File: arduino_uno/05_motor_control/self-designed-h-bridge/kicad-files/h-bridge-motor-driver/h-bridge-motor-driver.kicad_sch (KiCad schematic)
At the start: 21 parts, among them J1 Conn_01x05_Pin, J3 2601-3102, J4 2601-3102, Q1 IRF9540N, Q2 IRLIZ44N, Q3 IRF9540N, Q4 IRLIZ44N, Q5 BC547, Q6 BC547

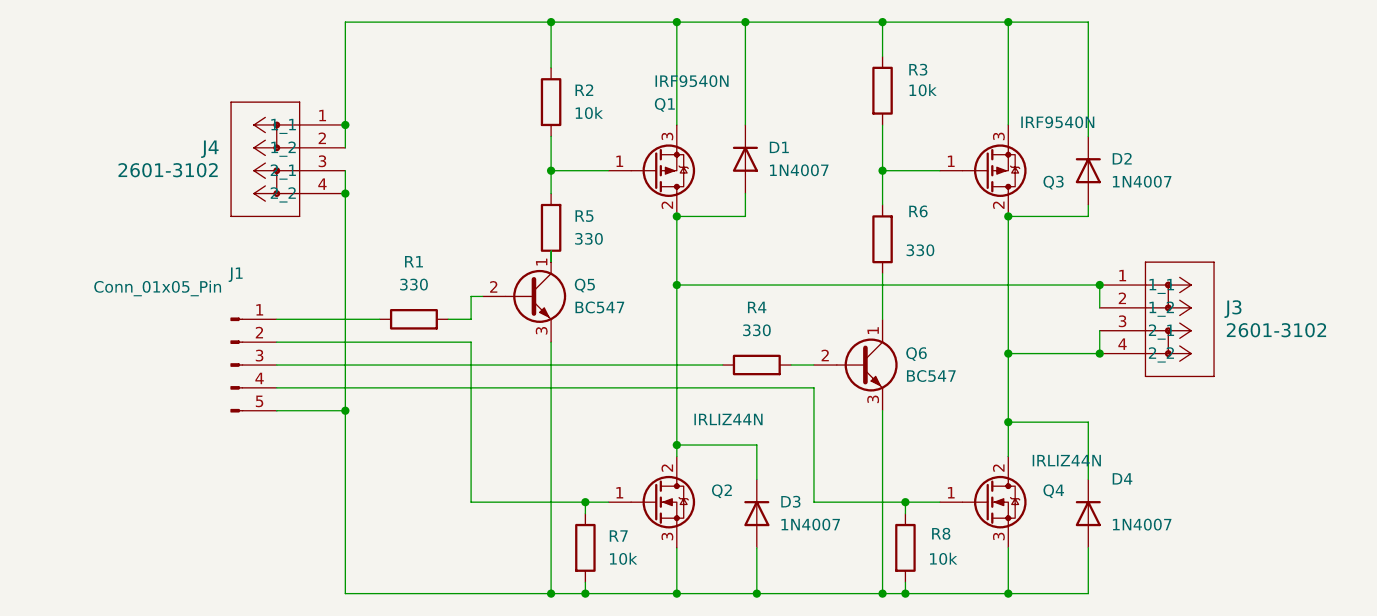
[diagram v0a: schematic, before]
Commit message: start routing
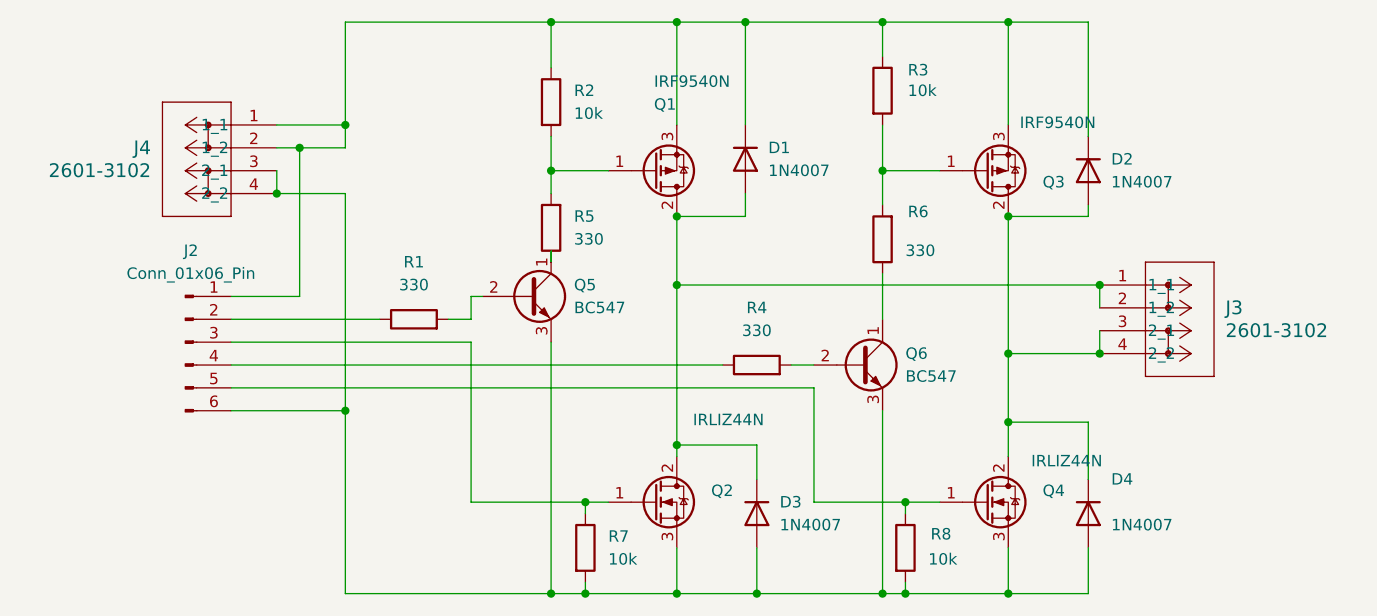
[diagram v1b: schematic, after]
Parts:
- removed J1: Conn_01x05_Pin, Connector_PinHeader_2.54mm:PinHeader_1x05_P2.54mm_Vertical, symbol Connector:Conn_01x05_Pin
- added J2: Conn_01x06_Pin, Connector_PinSocket_2.54mm:PinSocket_1x06_P2.54mm_Vertical, symbol Connector:Conn_01x06_Pin
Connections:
- net at D1.1 (K), D2.1 (K), J4.1 (1_1)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: now also J2.1 (Pin_1)
- net at Q4.1 (G), R8.1: now also J2.5 (Pin_5)
- net at D3.2 (A), D4.2 (A), J4.3 (2_1)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: now also J2.6 (Pin_6)
- net at Q2.1 (G), R7.1: now also J2.3 (Pin_3)
- net at R1.1: now also J2.2 (Pin_2)
- net at R4.1: now also J2.4 (Pin_4)
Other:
- moved on the sheet: J4
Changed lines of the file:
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@@
 	(paper "A4")
 	(junction
+		(at 66.04 60.96)
+		(diameter 0)
+		(color 0 0 0 0)
+	)
+	(junction
 		(at 97.79 100.33)
 		(diameter 0)
@@
 	)
 	(junction
-		(at 71.12 66.04)
-		(diameter 0)
-		(color 0 0 0 0)
-	)
-	(junction
 		(at 107.95 110.49)
 		(diameter 0)
@@
 	)
 	(junction
+		(at 63.5 66.04)
+		(diameter 0)
+		(color 0 0 0 0)
+	)
+	(junction
 		(at 107.95 93.98)
 		(diameter 0)
@@
 	(wire
 		(pts
+			(xy 58.42 87.63) (xy 123.19 87.63)
+		)
+		(stroke
+			(width 0)
+			(type default)
+		)
+	)
+	(wire
+		(pts
 			(xy 93.98 63.5) (xy 93.98 66.04)
 		)
@@
 	(wire
 		(pts
+			(xy 63.5 60.96) (xy 66.04 60.96)
+		)
+		(stroke
+			(width 0)
+			(type default)
+		)
+	)
+	(wire
+		(pts
 			(xy 85.09 77.47) (xy 85.09 80.01)
 		)
@@
 	(wire
 		(pts
+			(xy 63.5 58.42) (xy 71.12 58.42)
+		)
+		(stroke
+			(width 0)
+			(type default)
+		)
+	)
+	(wire
+		(pts
 			(xy 130.81 58.42) (xy 130.81 63.5)
 		)
@@
 	(wire
 		(pts
+			(xy 58.42 85.09) (xy 113.03 85.09)
+		)
+		(stroke
+			(width 0)
+			(type default)
+		)
+	)
+	(wire
+		(pts
 			(xy 130.81 63.5) (xy 137.16 63.5)
 		)
@@
 	(wire
 		(pts
+			(xy 58.42 82.55) (xy 85.09 82.55)
+		)
+		(stroke
+			(width 0)
+			(type default)
+		)
+	)
+	(wire
+		(pts
 			(xy 97.79 101.6) (xy 97.79 100.33)
 		)
@@
 	(wire
 		(pts
+			(xy 58.42 90.17) (xy 71.12 90.17)
+		)
+		(stroke
+			(width 0)
+			(type default)
+		)
+	)
+	(wire
+		(pts
 			(xy 85.09 100.33) (xy 97.79 100.33)
 		)
@@
 	(wire
 		(pts
+			(xy 63.5 66.04) (xy 71.12 66.04)
+		)
+		(stroke
+			(width 0)
+			(type default)
+		)
+	)
+	(wire
+		(pts
 			(xy 154.94 76.2) (xy 154.94 78.74)
 		)
@@
 	(wire
 		(pts
+			(xy 66.04 60.96) (xy 66.04 77.47)
+		)
+		(stroke
+			(width 0)
+			(type default)
+		)
+	)
+	(wire
+		(pts
 			(xy 116.84 110.49) (xy 107.95 110.49)
 		)
@@
 	(wire
 		(pts
-			(xy 63.5 90.17) (xy 71.12 90.17)
-		)
-		(stroke
-			(width 0)
-			(type default)
-		)
-	)
-	(wire
-		(pts
 			(xy 144.78 105.41) (xy 144.78 110.49)
 		)
@@
 	(wire
 		(pts
-			(xy 63.5 80.01) (xy 74.93 80.01)
-		)
-		(stroke
-			(width 0)
-			(type default)
-		)
-	)
-	(wire
-		(pts
-			(xy 63.5 85.09) (xy 113.03 85.09)
+			(xy 58.42 77.47) (xy 66.04 77.47)
 		)
 		(stroke
@@
 	(wire
 		(pts
-			(xy 71.12 58.42) (xy 71.12 60.96)
-		)
-		(stroke
-			(width 0)
-			(type default)
-		)
-	)
-	(wire
-		(pts
 			(xy 144.78 46.99) (xy 153.67 46.99)
 		)
@@
 	(wire
 		(pts
-			(xy 63.5 82.55) (xy 85.09 82.55)
-		)
-		(stroke
-			(width 0)
-			(type default)
-		)
-	)
-	(wire
-		(pts
 			(xy 116.84 93.98) (xy 107.95 93.98)
 		)
@@
 	(wire
 		(pts
-			(xy 71.12 63.5) (xy 71.12 66.04)
+			(xy 63.5 63.5) (xy 63.5 66.04)
 		)
 		(stroke
@@
 	(wire
 		(pts
+			(xy 71.12 60.96) (xy 71.12 58.42)
+		)
+		(stroke
+			(width 0)
+			(type default)
+		)
+	)
+	(wire
+		(pts
+			(xy 66.04 60.96) (xy 71.12 60.96)
+		)
+		(stroke
+			(width 0)
+			(type default)
+		)
+	)
+	(wire
+		(pts
 			(xy 144.78 110.49) (xy 133.35 110.49)
 		)
@@
 	(wire
 		(pts
-			(xy 63.5 87.63) (xy 123.19 87.63)
+			(xy 58.42 80.01) (xy 74.93 80.01)
 		)
 		(stroke
@@
 	)
 	(symbol
-		(lib_id "Connector:Conn_01x05_Pin")
-		(at 58.42 85.09 0)
-		(unit 1)
-		(exclude_from_sim no)
-		(in_bom yes)
-		(on_board yes)
-		(dnp no)
-		(property "Reference" "J1"
-			(at 59.055 74.93 0)
-			(effects
-				(font
-					(size 1.27 1.27)
-				)
-			)
-		)
-		(property "Value" "Conn_01x05_Pin"
-			(at 50.292 76.454 0)
-			(effects
-				(font
-					(size 1.27 1.27)
-				)
-			)
-		)
-		(property "Footprint" "Connector_PinHeader_2.54mm:PinHeader_1x05_P2.54mm_Vertical"
-			(at 58.42 85.09 0)
-			(effects
-				(font
-					(size 1.27 1.27)
-				)
-				(hide yes)
-			)
-		)
-		(property "Datasheet" "~"
-			(at 58.42 85.09 0)
-			(effects
-				(font
-					(size 1.27 1.27)
-				)
-				(hide yes)
-			)
-		)
-		(property "Description" "Generic connector, single row, 01x05, script generated"
-			(at 58.42 85.09 0)
-			(effects
-				(font
-					(size 1.27 1.27)
-				)
-				(hide yes)
-			)
-		)
-		(pin "2"
-		)
-		(pin "5"
-		)
-		(pin "3"
-		)
-		(pin "1"
-		)
-		(pin "4"
-		)
-		(instances
-			(project ""
-				(path "/c86b6916-14ad-4ba0-a61b-f63bb8896688"
-					(reference "J1")
-					(unit 1)
-				)
-			)
-		)
-	)
-	(symbol
 		(lib_id "Transistor_BJT:BC547")
 		(at 128.27 85.09 0)
@@
 		(lib_name "2601-3102_1")
 		(lib_id "Wago 2601-3102:2601-3102")
-		(at 71.12 58.42 0)
+		(at 63.5 58.42 0)
 		(mirror y)
 		(unit 1)
@@
 		(dnp no)
 		(property "Reference" "J4"
-			(at 57.15 60.9599 0)
+			(at 49.53 60.9599 0)
 			(effects
 				(font
@@
 		)
 		(property "Value" "2601-3102"
-			(at 57.15 63.4999 0)
+			(at 49.53 63.4999 0)
 			(effects
 				(font
@@
 		)
 		(property "Footprint" "WAGO 2601-3102:CONN2_2601-3102_WAG"
-			(at 71.12 58.42 0)
+			(at 63.5 58.42 0)
 			(effects
 				(font
@@
 		)
 		(property "Datasheet" "2601-3102"
-			(at 71.12 58.42 0)
+			(at 63.5 58.42 0)
 			(effects
 				(font
@@
 		)
 		(property "Description" ""
-			(at 71.12 58.42 0)
+			(at 63.5 58.42 0)
 			(effects
 				(font
@@
 					(unit 1)
 				)
+			)
+		)
+	)
+	(symbol
+		(lib_id "Connector:Conn_01x06_Pin")
+		(at 53.34 82.55 0)
+		(unit 1)
+		(exclude_from_sim no)
+		(in_bom yes)
+		(on_board yes)
+		(dnp no)
+		(fields_autoplaced yes)
+		(property "Reference" "J2"
+			(at 53.975 72.39 0)
+			(effects
+				(font
+					(size 1.27 1.27)
+				)
+			)
+		)
+		(property "Value" "Conn_01x06_Pin"
+			(at 53.975 74.93 0)
+			(effects
+				(font
+					(size 1.27 1.27)
+				)
+			)
+		)
+		(property "Footprint" "Connector_PinSocket_2.54mm:PinSocket_1x06_P2.54mm_Vertical"
+			(at 53.34 82.55 0)
+			(effects
+				(font
+					(size 1.27 1.27)
+				)
+				(hide yes)
+			)
+		)
+		(property "Datasheet" "~"
+			(at 53.34 82.55 0)
+			(effects
+				(font
+					(size 1.27 1.27)
+				)
+				(hide yes)
+			)
+		)
+		(property "Description" "Generic connector, single row, 01x06, script generated"
+			(at 53.34 82.55 0)
+			(effects
+				(font
+					(size 1.27 1.27)
+				)
+				(hide yes)
+			)
+		)
+		(pin "4"
+		)
+		(pin "2"
+		)
+		(pin "3"
+		)
+		(pin "1"
+		)
+		(pin "5"
+		)
+		(pin "6"
+		)
+		(instances
+			(project ""
+				(path "/c86b6916-14ad-4ba0-a61b-f63bb8896688"
+					(reference "J2")
+					(unit 1)
+				)
